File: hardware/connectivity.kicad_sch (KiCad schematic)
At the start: 13 parts, among them J1 GT-USB-7010ASV, J2 Pin Headers,2x20,SMD,P2.54mm,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, J3 SWD, U2 AMS1117-3.3

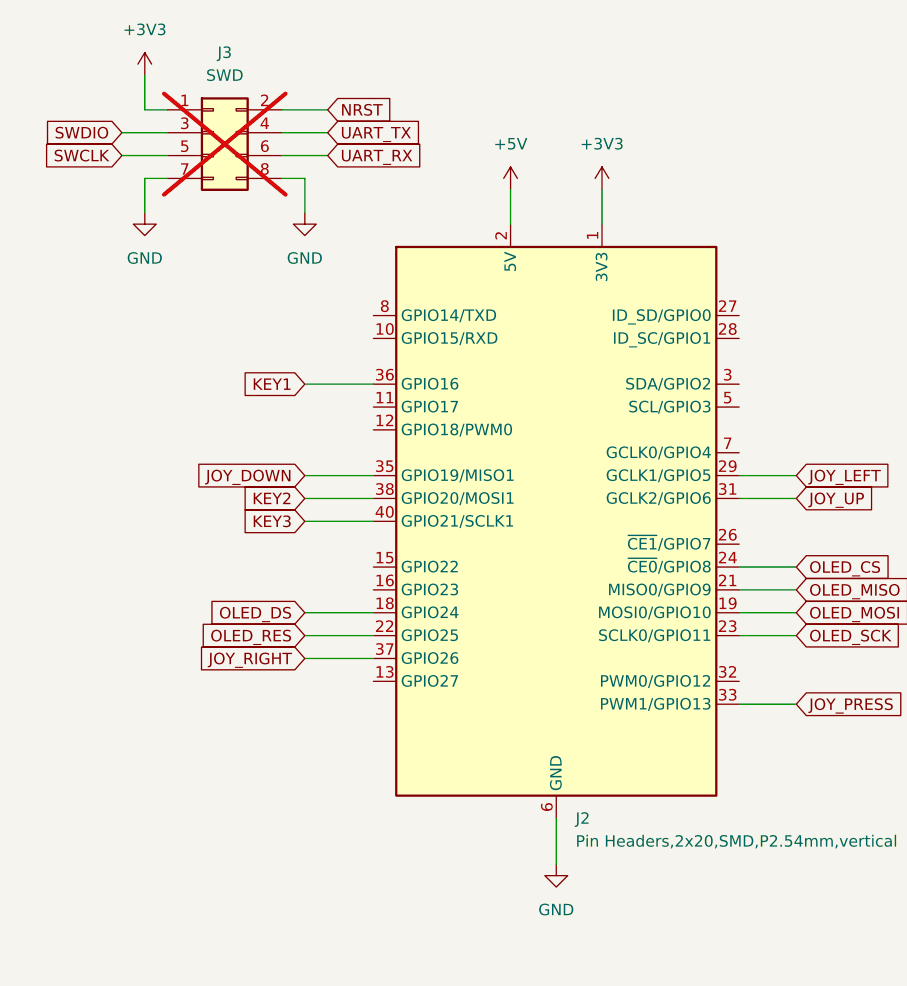
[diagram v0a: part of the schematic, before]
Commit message: Finished board
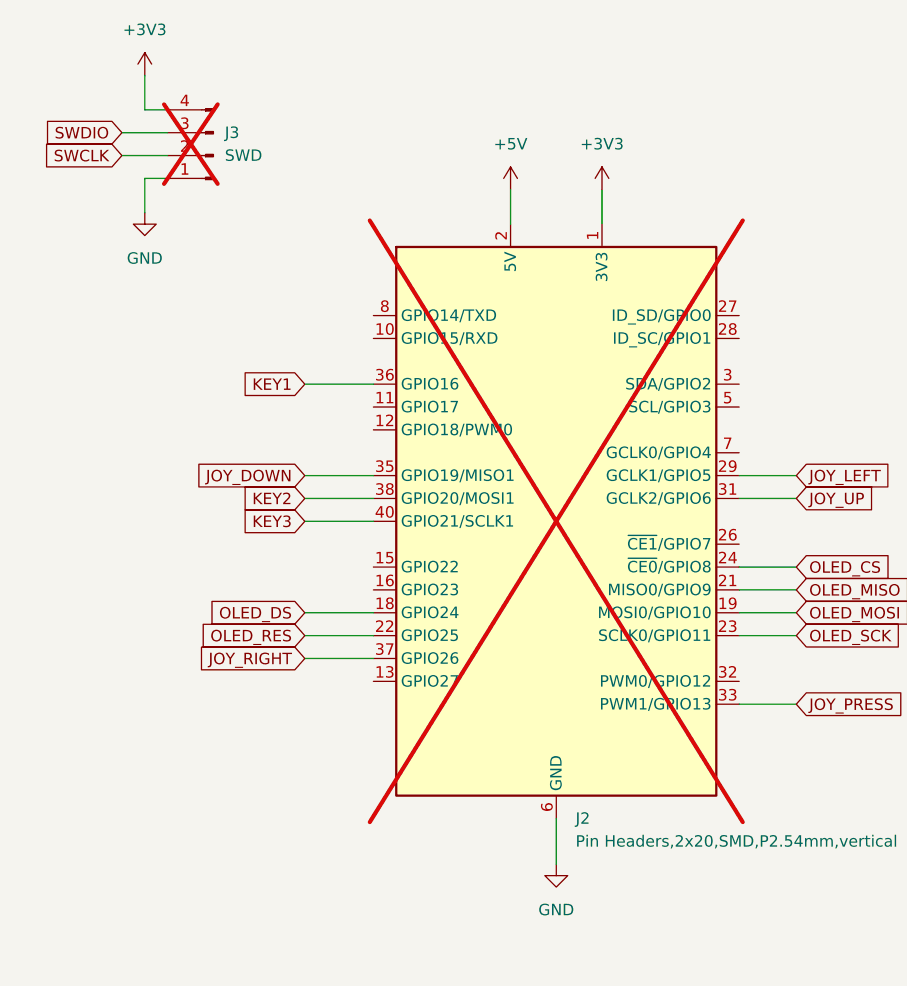
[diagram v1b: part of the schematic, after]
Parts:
- removed J3: SWD, Connector_PinHeader_2.54mm:PinHeader_2x04_P2.54mm_Horizontal, symbol Connector_Generic:Conn_02x04_Odd_Even
- added J3: SWD, Connector_PinHeader_2.54mm:PinHeader_1x04_P2.54mm_Horizontal, symbol Connector:Conn_01x04_Pin
- J2: footprint Connector_PinHeader_2.54mm:PinHeader_2x20_P2.54mm_Vertical_SMD -> Connector_PinHeader_2.54mm:PinHeader_2x20_P2.54mm_Vertical; now not fitted
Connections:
- net +3V3: now also J3.4 (Pin_4)
- net GND: now also J3.1 (Pin_1)
- net SWCLK: now also J3.2 (Pin_2)
- net SWDIO: now also J3.3 (Pin_3)

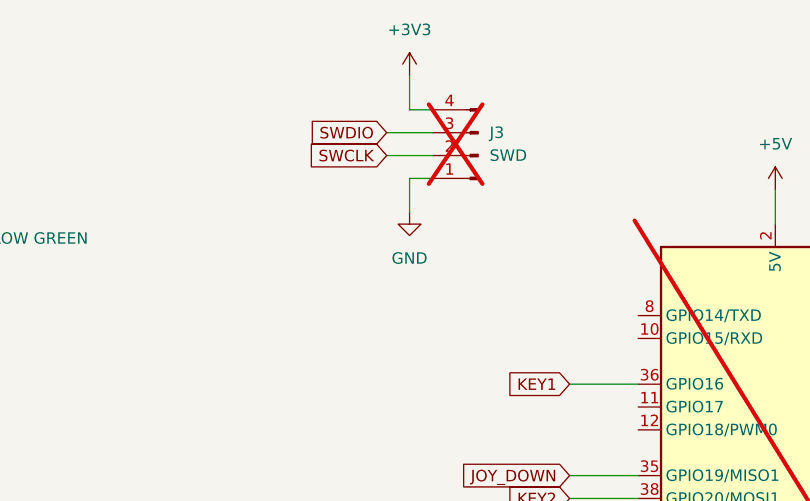
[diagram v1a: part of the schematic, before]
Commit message: Reorganized repo
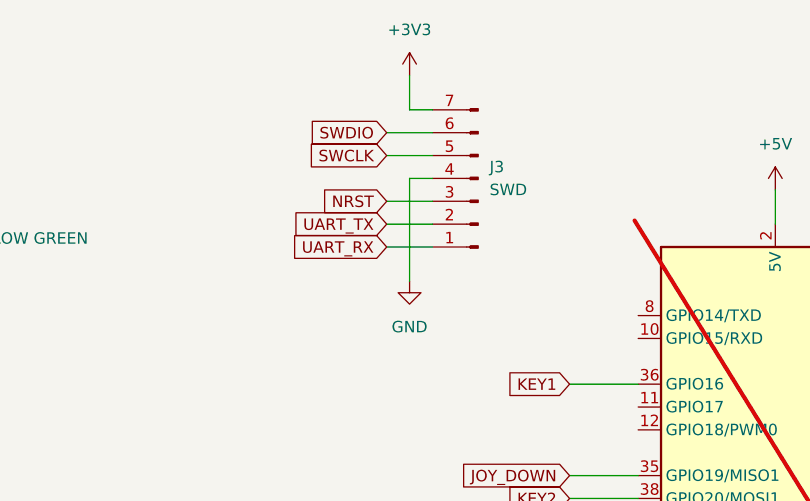
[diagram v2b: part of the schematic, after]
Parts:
- removed J3: SWD, Connector_PinHeader_2.54mm:PinHeader_1x04_P2.54mm_Horizontal, symbol Connector:Conn_01x04_Pin
- added J3: SWD, Connector_PinHeader_2.54mm:PinHeader_1x07_P2.54mm_Horizontal, symbol Connector:Conn_01x07_Pin
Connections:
- net +3V3: now also J3.7 (Pin_7)
- net GND: now also J3.4 (Pin_4)
- net SWCLK: now also J3.5 (Pin_5)
- net SWDIO: now also J3.6 (Pin_6)
- new net NRST: J3.3 (Pin_3)
- new net UART_RX: J3.1 (Pin_1)
- new net UART_TX: J3.2 (Pin_2)
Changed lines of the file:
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@@
 	(wire
 		(pts
-			(xy 160.02 58.42) (xy 160.02 62.23)
+			(xy 160.02 58.42) (xy 160.02 69.85)
 		)
 		(stroke
@@
 	(wire
 		(pts
+			(xy 157.48 60.96) (xy 162.56 60.96)
+		)
+		(stroke
+			(width 0)
+			(type default)
+		)
+	)
+	(wire
+		(pts
 			(xy 46.99 60.96) (xy 52.07 60.96)
 		)
@@
 	(wire
 		(pts
+			(xy 157.48 66.04) (xy 162.56 66.04)
+		)
+		(stroke
+			(width 0)
+			(type default)
+		)
+	)
+	(wire
+		(pts
 			(xy 36.83 60.96) (xy 41.91 60.96)
 		)
@@
 	(wire
 		(pts
+			(xy 157.48 63.5) (xy 162.56 63.5)
+		)
+		(stroke
+			(width 0)
+			(type default)
+		)
+	)
+	(wire
+		(pts
 			(xy 52.07 60.96) (xy 52.07 66.04)
 		)
@@
 		)
 	)
+	(global_label "UART_RX"
+		(shape input)
+		(at 157.48 66.04 180)
+		(fields_autoplaced yes)
+		(effects
+			(font
+				(size 1.27 1.27)
+			)
+			(justify right)
+		)
+		(property "Intersheetrefs" "${INTERSHEET_REFS}"
+			(at 146.391 66.04 0)
+			(effects
+				(font
+					(size 1.27 1.27)
+				)
+				(justify right)
+				(hide yes)
+			)
+		)
+	)
 	(global_label "KEY1"
 		(shape input)
@@
 		)
 	)
+	(global_label "NRST"
+		(shape input)
+		(at 157.48 60.96 180)
+		(fields_autoplaced yes)
+		(effects
+			(font
+				(size 1.27 1.27)
+			)
+			(justify right)
+		)
+		(property "Intersheetrefs" "${INTERSHEET_REFS}"
+			(at 149.7172 60.96 0)
+			(effects
+				(font
+					(size 1.27 1.27)
+				)
+				(justify right)
+				(hide yes)
+			)
+		)
+	)
 	(global_label "JOY_LEFT"
 		(shape input)
@@
 		)
 	)
+	(global_label "UART_TX"
+		(shape input)
+		(at 157.48 63.5 180)
+		(fields_autoplaced yes)
+		(effects
+			(font
+				(size 1.27 1.27)
+			)
+			(justify right)
+		)
+		(property "Intersheetrefs" "${INTERSHEET_REFS}"
+			(at 146.6934 63.5 0)
+			(effects
+				(font
+					(size 1.27 1.27)
+				)
+				(justify right)
+				(hide yes)
+			)
+		)
+	)
 	(global_label "KEY3"
 		(shape input)
@@
 	(symbol
 		(lib_id "power:GND")
-		(at 160.02 62.23 0)
+		(at 160.02 69.85 0)
 		(unit 1)
 		(exclude_from_sim no)
@@
 		(fields_autoplaced yes)
 		(property "Reference" "#PWR029"
-			(at 160.02 68.58 0)
+			(at 160.02 76.2 0)
 			(effects
 				(font
@@
 		)
 		(property "Value" "GND"
-			(at 160.02 67.31 0)
+			(at 160.02 74.93 0)
 			(effects
 				(font
@@
 		)
 		(property "Footprint" ""
-			(at 160.02 62.23 0)
+			(at 160.02 69.85 0)
 			(effects
 				(font
@@
 		)
 		(property "Datasheet" ""
-			(at 160.02 62.23 0)
+			(at 160.02 69.85 0)
 			(effects
 				(font
@@
 		)
 		(property "Description" "Power symbol creates a global label with name \"GND\" , ground"
-			(at 160.02 62.23 0)
+			(at 160.02 69.85 0)
 			(effects
 				(font
@@
 	)
 	(symbol
-		(lib_id "Connector:Conn_01x04_Pin")
-		(at 167.64 55.88 180)
-		(unit 1)
-		(exclude_from_sim no)
-		(in_bom yes)
-		(on_board yes)
-		(dnp yes)
-		(property "Reference" "J3"
-			(at 168.91 53.3399 0)
-			(effects
-				(font
-					(size 1.27 1.27)
-				)
-				(justify right)
-			)
-		)
-		(property "Value" "SWD"
-			(at 168.91 55.8799 0)
-			(effects
-				(font
-					(size 1.27 1.27)
-				)
-				(justify right)
-			)
-		)
-		(property "Footprint" "Connector_PinHeader_2.54mm:PinHeader_1x04_P2.54mm_Horizontal"
-			(at 166.624 39.116 0)
-			(effects
-				(font
-					(size 1.27 1.27)
-				)
-				(hide yes)
-			)
-		)
-		(property "Datasheet" "~"
-			(at 167.64 55.88 0)
-			(effects
-				(font
-					(size 1.27 1.27)
-				)
-				(hide yes)
-			)
-		)
-		(property "Description" "Generic connector, single row, 01x04, script generated"
-			(at 167.64 55.88 0)
-			(effects
-				(font
-					(size 1.27 1.27)
-				)
-				(hide yes)
-			)
-		)
-		(pin "3"
-		)
-		(pin "2"
-		)
-		(pin "1"
-		)
-		(pin "4"
-		)
-		(instances
-			(project ""
-				(path "/301ddcee-4740-4eda-b689-6f23930b1798/318b2e69-26c4-459c-82f8-99b530565fe2"
-					(reference "J3")
-					(unit 1)
-				)
-			)
-		)
-	)
-	(symbol
 		(lib_id "power:+3V3")
 		(at 160.02 46.99 0)
@@
 					(unit 1)
 				)
+			)
+		)
+	)
+	(symbol
+		(lib_id "Connector:Conn_01x07_Pin")
+		(at 167.64 58.42 180)
+		(unit 1)
+		(exclude_from_sim no)
+		(in_bom yes)
+		(on_board yes)
+		(dnp no)
+		(fields_autoplaced yes)
+		(property "Reference" "J3"
+			(at 168.91 57.1499 0)
+			(effects
+				(font
+					(size 1.27 1.27)
+				)
+				(justify right)
+			)
+		)
+		(property "Value" "SWD"
+			(at 168.91 59.6899 0)
+			(effects
+				(font
+					(size 1.27 1.27)
+				)
+				(justify right)
+			)
+		)
+		(property "Footprint" "Connector_PinHeader_2.54mm:PinHeader_1x07_P2.54mm_Horizontal"
+			(at 167.64 58.42 0)
+			(effects
+				(font
+					(size 1.27 1.27)
+				)
+				(hide yes)
+			)
+		)
+		(property "Datasheet" "~"
+			(at 167.64 58.42 0)
+			(effects
+				(font
+					(size 1.27 1.27)
+				)
+				(hide yes)
+			)
+		)
+		(property "Description" "Generic connector, single row, 01x07, script generated"
+			(at 167.64 58.42 0)
+			(effects
+				(font
+					(size 1.27 1.27)
+				)
+				(hide yes)
+			)
+		)
+		(property "LCSC Part #" ""
+			(at 167.64 58.42 0)
+			(effects
+				(font
+					(size 1.27 1.27)
+				)
+				(hide yes)
+			)
+		)
+		(pin "1"
+		)
+		(pin "2"
+		)
+		(pin "3"
+		)
+		(pin "4"
+		)
+		(pin "5"
+		)
+		(pin "6"
+		)
+		(pin "7"
+		)
+		(instances
+			(project ""
+				(path "/301ddcee-4740-4eda-b689-6f23930b1798/318b2e69-26c4-459c-82f8-99b530565fe2"
+					(reference "J3")
+					(unit 1)
+				)
